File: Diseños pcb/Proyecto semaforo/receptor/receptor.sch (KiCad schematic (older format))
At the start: 7 parts, among them J1 Conn_01x03_Male, Q1 2N3904, Q2 2N3904

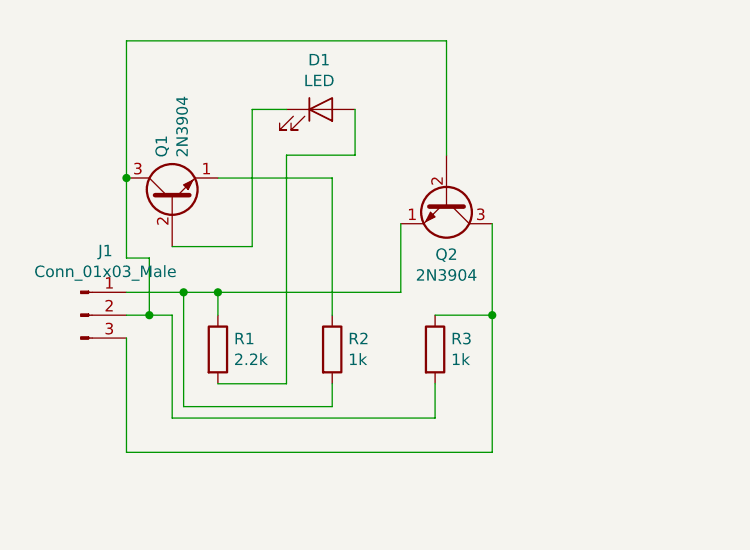
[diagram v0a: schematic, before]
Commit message: Diseños PCB actualizados
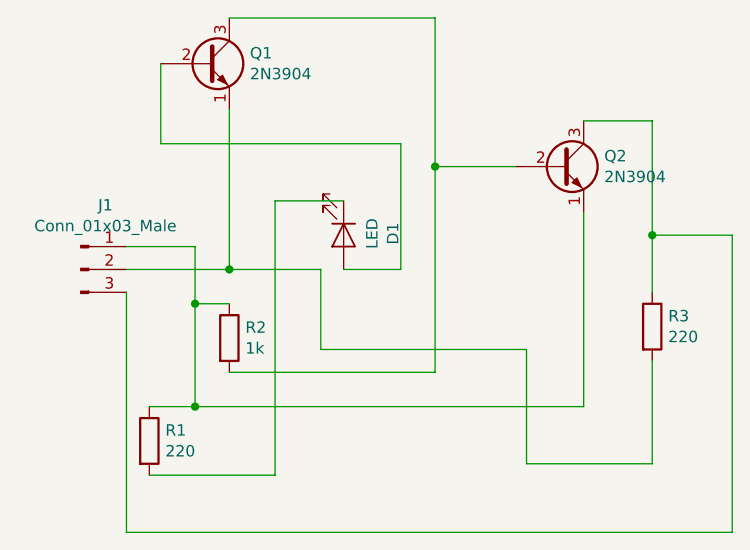
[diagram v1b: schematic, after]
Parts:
- J1: footprint Connector_JST:JST_NV_B03P-NV_1x03_P5.00mm_Vertical -> Connector_JST:JST_EH_B3B-EH-A_1x03_P2.50mm_Vertical
- R1: value 2.2k -> 220
- R3: value 1k -> 220; footprint Resistor_THT:R_Axial_DIN0309_L9.0mm_D3.2mm_P12.70mm_Horizontal -> Resistor_THT:R_Axial_DIN0411_L9.9mm_D3.6mm_P12.70mm_Horizontal
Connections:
- net at R2.1: now also J1.1 (Pin_1), Q2.1 (E), R1.1; no longer Q1.1 (E)
- net at D1.1 (K): now also R1.2; no longer Q1.2 (B)
- net at J1.2 (Pin_2), R3.2: now also Q1.1 (E); no longer Q1.3 (C), Q2.2 (B)
- net at D1.2 (A): now also Q1.2 (B); no longer R1.2
- new net: Q1.3 (C), Q2.2 (B), R2.2
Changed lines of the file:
@@
 EESchema Schematic File Version 4
+LIBS:receptor-cache
 EELAYER 30 0
 EELAYER END
@@
 $EndDescr
 $Comp
-L Transistor_BJT:2N3904 Q1
-U 1 1 5D7D1409
-P 1550 1350
-F 0 "Q1" H 1740 1396 50  0000 L CNN
-F 1 "2N3904" H 1740 1305 50  0000 L CNN
-F 2 "Package_TO_SOT_THT:TO-92_Inline" H 1750 1275 50  0001 L CIN
-F 3 "https://www.fairchildsemi.com/datasheets/2N/2N3904.pdf" H 1550 1350 50  0001 L CNN
-	1    1550 1350
-	0    -1   -1   0
-$EndComp
-$Comp
-L Transistor_BJT:2N3904 Q2
-U 1 1 5D7D1A0F
-P 2750 1350
-F 0 "Q2" V 2985 1350 50  0000 C CNN
-F 1 "2N3904" V 3076 1350 50  0000 C CNN
-F 2 "Package_TO_SOT_THT:TO-92_Inline" H 2950 1275 50  0001 L CIN
-F 3 "https://www.fairchildsemi.com/datasheets/2N/2N3904.pdf" H 2750 1350 50  0001 L CNN
-	1    2750 1350
-	0    1    1    0
+L Connector:Conn_01x03_Male J1
+U 1 1 5D801336
+P 1150 1650
+F 0 "J1" H 1258 1931 50  0000 C CNN
+F 1 "Conn_01x03_Male" H 1258 1840 50  0000 C CNN
+F 2 "Connector_JST:JST_EH_B3B-EH-A_1x03_P2.50mm_Vertical" H 1150 1650 50  0001 C CNN
+F 3 "~" H 1150 1650 50  0001 C CNN
+	1    1150 1650
+	1    0    0    -1
 $EndComp
 $Comp
 L Device:R R1
-U 1 1 5D7D1EB4
-P 1750 2000
-F 0 "R1" H 1820 2046 50  0000 L CNN
-F 1 "2.2k" H 1820 1955 50  0000 L CNN
-F 2 "Resistor_THT:R_Axial_DIN0309_L9.0mm_D3.2mm_P12.70mm_Horizontal" V 1680 2000 50  0001 C CNN
-F 3 "~" H 1750 2000 50  0001 C CNN
-	1    1750 2000
+U 1 1 5D8017ED
+P 1450 2400
+F 0 "R1" H 1520 2446 50  0000 L CNN
+F 1 "220" H 1520 2355 50  0000 L CNN
+F 2 "Resistor_THT:R_Axial_DIN0309_L9.0mm_D3.2mm_P12.70mm_Horizontal" V 1380 2400 50  0001 C CNN
+F 3 "~" H 1450 2400 50  0001 C CNN
+	1    1450 2400
 	1    0    0    -1
 $EndComp
 $Comp
 L Device:R R2
-U 1 1 5D7D21E5
-P 2250 2000
-F 0 "R2" H 2320 2046 50  0000 L CNN
-F 1 "1k" H 2320 1955 50  0000 L CNN
-F 2 "Resistor_THT:R_Axial_DIN0309_L9.0mm_D3.2mm_P12.70mm_Horizontal" V 2180 2000 50  0001 C CNN
-F 3 "~" H 2250 2000 50  0001 C CNN
-	1    2250 2000
+U 1 1 5D801A73
+P 1800 1950
+F 0 "R2" H 1870 1996 50  0000 L CNN
+F 1 "1k" H 1870 1905 50  0000 L CNN
+F 2 "Resistor_THT:R_Axial_DIN0309_L9.0mm_D3.2mm_P12.70mm_Horizontal" V 1730 1950 50  0001 C CNN
+F 3 "~" H 1800 1950 50  0001 C CNN
+	1    1800 1950
 	1    0    0    -1
 $EndComp
 $Comp
 L Device:R R3
-U 1 1 5D7D2562
-P 2700 2000
-F 0 "R3" H 2770 2046 50  0000 L CNN
-F 1 "1k" H 2770 1955 50  0000 L CNN
-F 2 "Resistor_THT:R_Axial_DIN0309_L9.0mm_D3.2mm_P12.70mm_Horizontal" V 2630 2000 50  0001 C CNN
-F 3 "~" H 2700 2000 50  0001 C CNN
-	1    2700 2000
+U 1 1 5D8021E1
+P 3650 1900
+F 0 "R3" H 3720 1946 50  0000 L CNN
+F 1 "220" H 3720 1855 50  0000 L CNN
+F 2 "Resistor_THT:R_Axial_DIN0411_L9.9mm_D3.6mm_P12.70mm_Horizontal" V 3580 1900 50  0001 C CNN
+F 3 "~" H 3650 1900 50  0001 C CNN
+	1    3650 1900
+	1    0    0    -1
+$EndComp
+$Comp
+L Transistor_BJT:2N3904 Q1
+U 1 1 5D8023FF
+P 1700 750
+F 0 "Q1" H 1890 796 50  0000 L CNN
+F 1 "2N3904" H 1890 705 50  0000 L CNN
+F 2 "Package_TO_SOT_THT:TO-92_Inline" H 1900 675 50  0001 L CIN
+F 3 "https://www.fairchildsemi.com/datasheets/2N/2N3904.pdf" H 1700 750 50  0001 L CNN
+	1    1700 750
+	1    0    0    -1
+$EndComp
+$Comp
+L Transistor_BJT:2N3904 Q2
+U 1 1 5D8027DA
+P 3250 1200
+F 0 "Q2" H 3440 1246 50  0000 L CNN
+F 1 "2N3904" H 3440 1155 50  0000 L CNN
+F 2 "Package_TO_SOT_THT:TO-92_Inline" H 3450 1125 50  0001 L CIN
+F 3 "https://www.fairchildsemi.com/datasheets/2N/2N3904.pdf" H 3250 1200 50  0001 L CNN
+	1    3250 1200
 	1    0    0    -1
 $EndComp
 $Comp
 L Device:LED D1
-U 1 1 5D7D2810
-P 2200 950
-F 0 "D1" H 2193 1166 50  0000 C CNN
-F 1 "LED" H 2193 1075 50  0000 C CNN
-F 2 "LED_THT:LED_D5.0mm" H 2200 950 50  0001 C CNN
-F 3 "~" H 2200 950 50  0001 C CNN
-	1    2200 950
-	1    0    0    -1
-$EndComp
-$Comp
-L Connector:Conn_01x03_Male J1
-U 1 1 5D7D6512
-P 1150 1850
-F 0 "J1" H 1258 2131 50  0000 C CNN
-F 1 "Conn_01x03_Male" H 1258 2040 50  0000 C CNN
-F 2 "Connector_JST:JST_NV_B03P-NV_1x03_P5.00mm_Vertical" H 1150 1850 50  0001 C CNN
-F 3 "~" H 1150 1850 50  0001 C CNN
-	1    1150 1850
-	1    0    0    -1
+U 1 1 5D805AB6
+P 2300 1500
+F 0 "D1" H 2293 1716 50  0000 C CNN
+F 1 "LED" H 2293 1625 50  0000 C CNN
+F 2 "LED_THT:LED_D5.0mm" H 2300 1500 50  0001 C CNN
+F 3 "~" H 2300 1500 50  0001 C CNN
+	1    2300 1500
+	0    1    1    0
 $EndComp
 Wire Wire Line
-	1350 1750 1600 1750
+	1350 1550 1650 1550
 Wire Wire Line
-	1750 1750 1750 1850
+	1650 1550 1650 1800
 Wire Wire Line
-	1750 2150 2050 2150
+	1650 2250 1450 2250
 Wire Wire Line
-	2050 2150 2050 1150
+	1450 2550 2000 2550
 Wire Wire Line
-	2050 1150 2350 1150
+	2000 2550 2000 1350
 Wire Wire Line
-	2350 1150 2350 950
+	2000 1350 2300 1350
 Wire Wire Line
-	1600 1750 1600 2250
+	1500 750  1500 1100
 Wire Wire Line
-	1600 2250 2250 2250
+	1500 1100 2550 1100
 Wire Wire Line
-	2250 2250 2250 2150
-Connection ~ 1600 1750
+	2550 1100 2550 1650
 Wire Wire Line
-	1600 1750 1750 1750
+	2550 1650 2300 1650
 Wire Wire Line
-	1350 1850 1450 1850
+	1800 950  1800 1650
 Wire Wire Line
-	1550 1850 1550 2300
+	1800 1650 1350 1650
 Wire Wire Line
-	1550 2300 2700 2300
+	1800 550  2700 550
 Wire Wire Line
-	2700 2300 2700 2150
+	2700 550  2700 1200
 Wire Wire Line
-	1750 1250 2250 1250
+	2700 2100 1800 2100
 Wire Wire Line
-	2250 1250 2250 1850
+	1650 1800 1800 1800
+Connection ~ 1650 1800
 Wire Wire Line
-	1550 1550 1900 1550
+	1650 1800 1650 2250
 Wire Wire Line
-	1900 1550 1900 950
+	3050 1200 2700 1200
+Connection ~ 2700 1200
 Wire Wire Line
-	1900 950  2050 950
+	2700 1200 2700 2100
 Wire Wire Line
-	1350 1250 1350 1600
+	1650 2250 3350 2250
 Wire Wire Line
-	1350 1600 1450 1600
+	3350 2250 3350 1400
+Connection ~ 1650 2250
 Wire Wire Line
-	1450 1600 1450 1850
-Connection ~ 1450 1850
+	3350 1000 3650 1000
 Wire Wire Line
-	1450 1850 1550 1850
+	3650 1000 3650 1500
 Wire Wire Line
-	2950 1450 2950 1850
+	1800 1650 2200 1650
 Wire Wire Line
-	2950 2450 1350 2450
+	2200 1650 2200 2000
 Wire Wire Line
-	1350 2450 1350 1950
+	2200 2000 3100 2000
 Wire Wire Line
-	1350 1250 1350 650
+	3100 2000 3100 2500
 Wire Wire Line
-	1350 650  2750 650
+	3100 2500 3650 2500
 Wire Wire Line
-	2750 650  2750 1150
-Connection ~ 1350 1250
+	3650 2500 3650 2050
+Connection ~ 1800 1650
 Wire Wire Line
-	1750 1750 2550 1750
+	1350 1750 1350 2800
 Wire Wire Line
-	2550 1750 2550 1450
-Connection ~ 1750 1750
+	1350 2800 4000 2800
 Wire Wire Line
-	2700 1850 2950 1850
-Connection ~ 2950 1850
+	4000 2800 4000 1500
 Wire Wire Line
-	2950 1850 2950 2450
+	4000 1500 3650 1500
+Connection ~ 3650 1500
+Wire Wire Line
+	3650 1500 3650 1750
 $EndSCHEMATC
